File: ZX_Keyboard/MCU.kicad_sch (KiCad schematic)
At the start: 19 parts, among them J1 DEBUG, J2 DBG_UART, SW1 RESET, U1 STM32F105R8Tx, Y1 Crystal

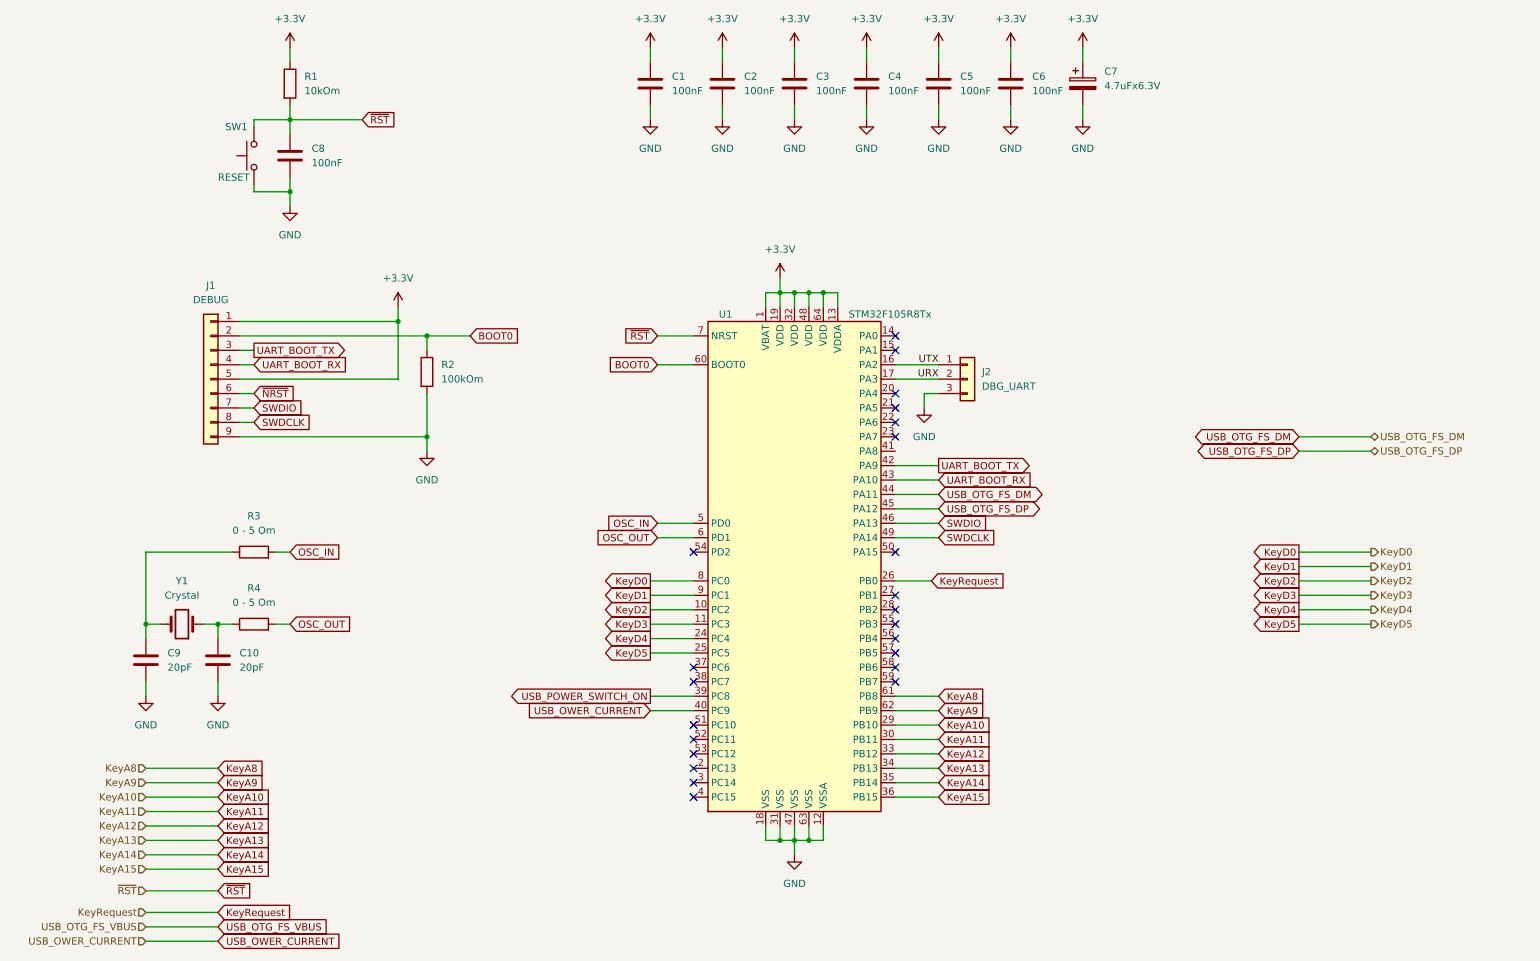
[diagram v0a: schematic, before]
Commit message: improve zx_keyboard schematic
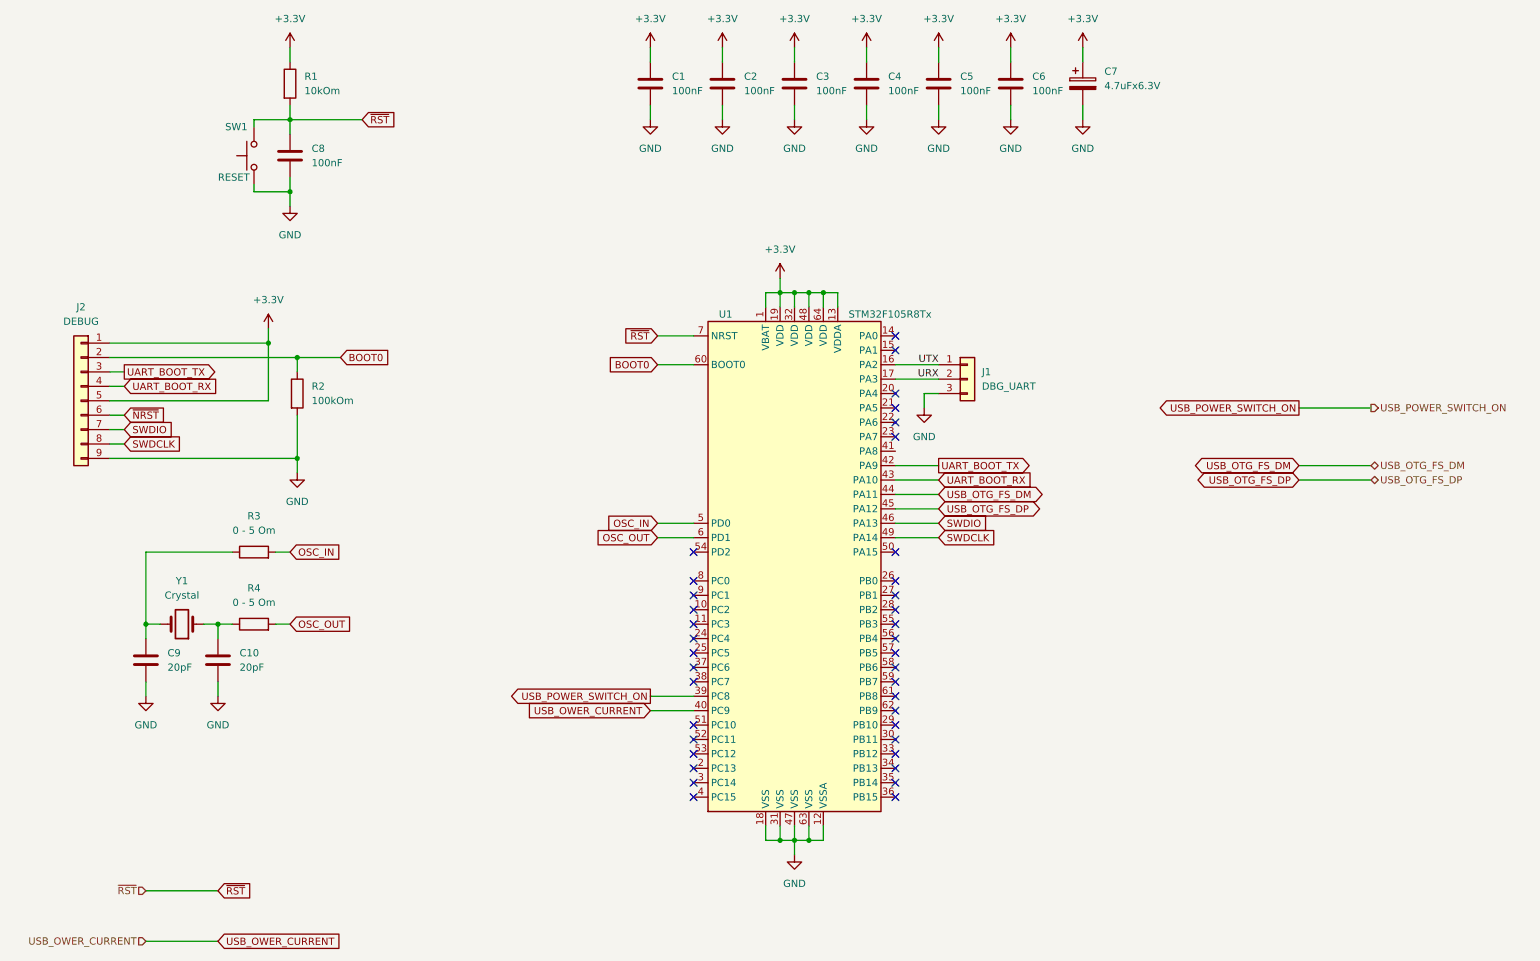
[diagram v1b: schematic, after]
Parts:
- renumbered J2 to J1, J1 to J2
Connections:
- net KeyA10: no longer names the net of U1.29 (PB10)
- net KeyA11: no longer names the net of U1.30 (PB11)
- net KeyA12: no longer names the net of U1.33 (PB12)
- net KeyA13: no longer names the net of U1.34 (PB13)
- net KeyA14: no longer names the net of U1.35 (PB14)
- net KeyA15: no longer names the net of U1.36 (PB15)
- net KeyA8: no longer names the net of U1.61 (PB8)
- net KeyA9: no longer names the net of U1.62 (PB9)
- net KeyD0: no longer names the net of U1.8 (PC0)
- net KeyD1: no longer names the net of U1.9 (PC1)
- net KeyD2: no longer names the net of U1.10 (PC2)
- net KeyD3: no longer names the net of U1.11 (PC3)
- net KeyD4: no longer names the net of U1.24 (PC4)
- net KeyD5: no longer names the net of U1.25 (PC5)
- net KeyRequest: no longer names the net of U1.26 (PB0)
- no-connect marks 23 -> 38
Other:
- moved on the sheet: J2, R2
